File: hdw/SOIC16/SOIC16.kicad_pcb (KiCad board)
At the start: 2 copper layers, 21.6 x 16.5 mm, 3 parts, among them J16 SOIC16-P01-P08, J17 SOIC16-P09-P16, U5 CH340C

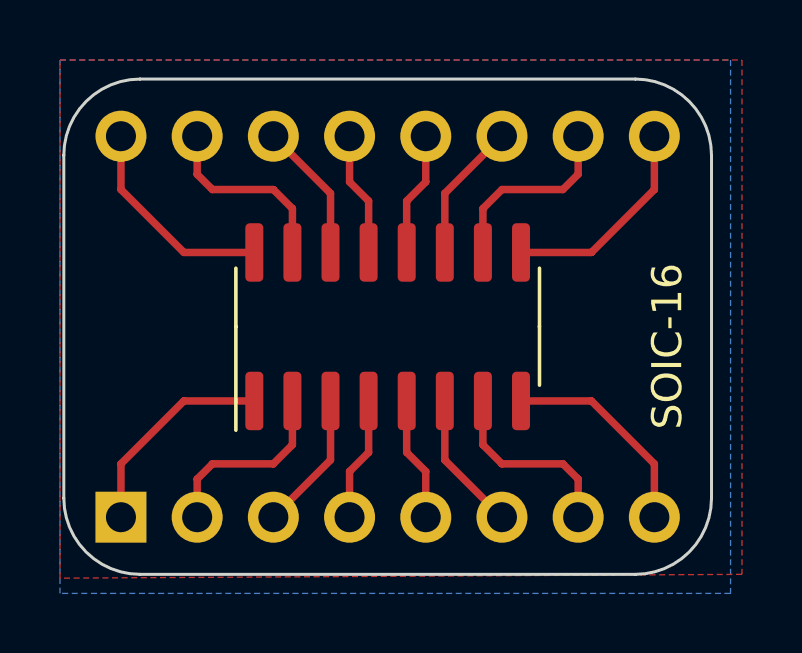
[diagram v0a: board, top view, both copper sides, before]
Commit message: Save changes at: 1736073146
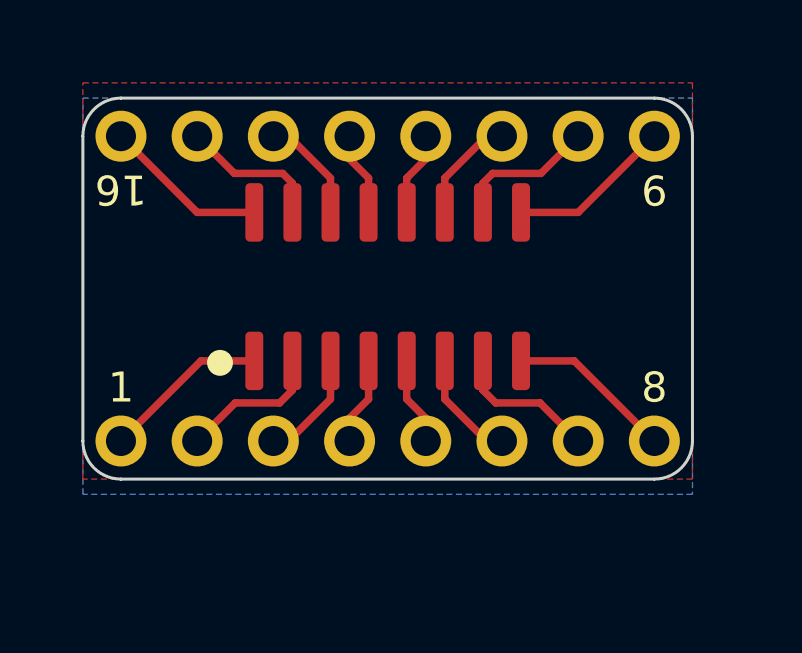
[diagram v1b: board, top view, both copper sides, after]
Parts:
- moved J16 2.54 mm to (96.5, 109.2)
- moved U5 1.33 mm to (105.4, 104.1)
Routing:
- net SOIC16-P16: track 7.09 -> 5.50 mm
- net SOIC16-P09: track 7.09 -> 5.50 mm
- net SOIC16-P15: track 6.38 -> 4.80 mm
- net SOIC16-P10: track 6.38 -> 4.80 mm
- net SOIC16-P08: track 7.09 -> 5.55 mm
- net SOIC16-P01: track 7.09 -> 5.55 mm
- net SOIC16-P07: track 6.38 -> 4.85 mm
- net SOIC16-P02: track 6.38 -> 4.85 mm
- net SOIC16-P13: track 4.14 -> 2.80 mm
- net SOIC16-P12: track 4.14 -> 2.80 mm
- net SOIC16-P04: track 4.14 -> 2.93 mm
- net SOIC16-P05: track 4.14 -> 2.93 mm
- net SOIC16-P11: track 4.66 -> 3.63 mm
- net SOIC16-P14: track 4.66 -> 3.63 mm
- net SOIC16-P06: track 4.66 -> 3.76 mm
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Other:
- board size 21.6 x 16.5 mm -> 20.3 x 12.7 mm
- board text added: "1"
- board text added: "16"
- board text added: "8"
- board text added: "9"
